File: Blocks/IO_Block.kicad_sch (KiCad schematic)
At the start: 0 parts

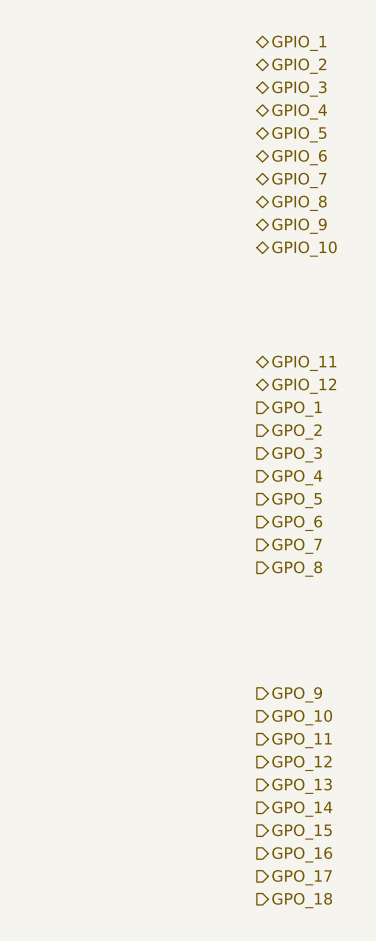
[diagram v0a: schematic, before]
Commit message: something
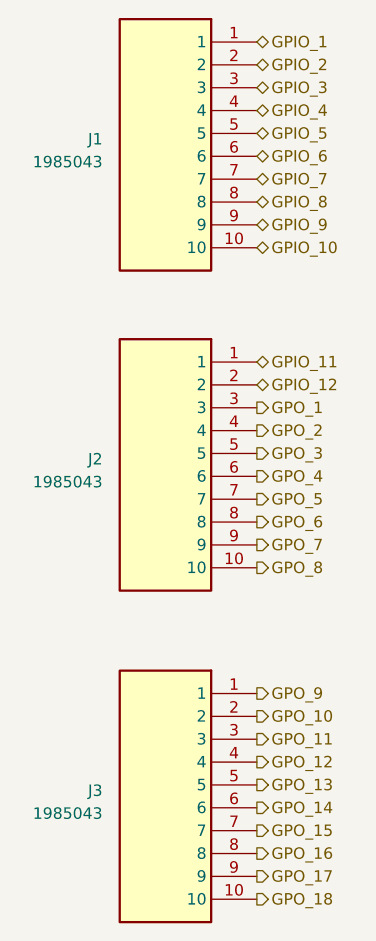
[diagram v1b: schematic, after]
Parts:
- added J1, J2, J3: 1985043, 1985043:1985043, symbol 1985043.kicad_sym:1985043
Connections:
- net GPIO_1: now also J1.1
- net GPIO_10: now also J1.10
- net GPIO_11: now also J2.1
- net GPIO_12: now also J2.2
- net GPIO_2: now also J1.2
- net GPIO_3: now also J1.3
- net GPIO_4: now also J1.4
- net GPIO_5: now also J1.5
- net GPIO_6: now also J1.6
- net GPIO_7: now also J1.7
- net GPIO_8: now also J1.8
- net GPIO_9: now also J1.9
- net GPO_1: now also J2.3
- net GPO_10: now also J3.2
- net GPO_11: now also J3.3
- net GPO_12: now also J3.4
- net GPO_13: now also J3.5
- net GPO_14: now also J3.6
- net GPO_15: now also J3.7
- net GPO_16: now also J3.8
- net GPO_17: now also J3.9
- net GPO_18: now also J3.10
- net GPO_2: now also J2.4
- net GPO_3: now also J2.5
- net GPO_4: now also J2.6
- net GPO_5: now also J2.7
- net GPO_6: now also J2.8
- net GPO_7: now also J2.9
- net GPO_8: now also J2.10
- net GPO_9: now also J3.1
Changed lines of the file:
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@@
     (effects (font (size 1.27 1.27)) (justify left))
   )
+  (symbol (lib_id "1985043.kicad_sym:1985043") (at 86.36 130.81 0) (mirror y) (unit 1)
+    (in_bom yes) (on_board yes) (dnp no)
+    (property "Reference" "J3" (at 69.215 141.605 0)
+      (effects (font (size 1.27 1.27)) (justify left))
+    )
+    (property "Value" "1985043" (at 69.215 144.145 0)
+      (effects (font (size 1.27 1.27)) (justify left))
+    )
+    (property "Footprint" "1985043:1985043" (at 69.85 225.73 0)
+      (effects (font (size 1.27 1.27)) (justify left top) hide)
+    )
+    (property "Datasheet" "https://www.phoenixcontact.com/online/portal/us/?uri=pxc-oc-itemdetail:pid=1985043&library=usen&pcck=P-11-01-05&tab=1&selectedCategory=ALL" (at 69.85 325.73 0)
+      (effects (font (size 1.27 1.27)) (justify left top) hide)
+    )
+    (property "Height" "13.1" (at 69.85 525.73 0)
+      (effects (font (size 1.27 1.27)) (justify left top) hide)
+    )
+    (property "Mouser Part Number" "651-1985043" (at 69.85 625.73 0)
+      (effects (font (size 1.27 1.27)) (justify left top) hide)
+    )
+    (property "Mouser Price/Stock" "https://www.mouser.co.uk/ProductDetail/Phoenix-Contact/1985043?qs=gjk32EaArKJe8oo3YkKpaw%3D%3D" (at 69.85 725.73 0)
+      (effects (font (size 1.27 1.27)) (justify left top) hide)
+    )
+    (property "Manufacturer_Name" "Phoenix Contact" (at 69.85 825.73 0)
+      (effects (font (size 1.27 1.27)) (justify left top) hide)
+    )
+    (property "Manufacturer_Part_Number" "1985043" (at 69.85 925.73 0)
+      (effects (font (size 1.27 1.27)) (justify left top) hide)
+    )
+    (pin "1")
+    (pin "10")
+    (pin "2")
+    (pin "3")
+    (pin "4")
+    (pin "5")
+    (pin "6")
+    (pin "7")
+    (pin "8")
+    (pin "9")
+    (instances
+      (project "PLC-CIM"
+        (path "/98f81d77-8880-491b-a7cf-4c27e2d73edf/ef38368d-af5e-44c5-8106-4a2f4dcc6c35"
+          (reference "J3") (unit 1)
+        )
+      )
+    )
+  )
+  (symbol (lib_id "1985043.kicad_sym:1985043") (at 86.36 58.42 0) (mirror y) (unit 1)
+    (in_bom yes) (on_board yes) (dnp no)
+    (property "Reference" "J1" (at 69.215 69.215 0)
+      (effects (font (size 1.27 1.27)) (justify left))
+    )
+    (property "Value" "1985043" (at 69.215 71.755 0)
+      (effects (font (size 1.27 1.27)) (justify left))
+    )
+    (property "Footprint" "1985043:1985043" (at 69.85 153.34 0)
+      (effects (font (size 1.27 1.27)) (justify left top) hide)
+    )
+    (property "Datasheet" "https://www.phoenixcontact.com/online/portal/us/?uri=pxc-oc-itemdetail:pid=1985043&library=usen&pcck=P-11-01-05&tab=1&selectedCategory=ALL" (at 69.85 253.34 0)
+      (effects (font (size 1.27 1.27)) (justify left top) hide)
+    )
+    (property "Height" "13.1" (at 69.85 453.34 0)
+      (effects (font (size 1.27 1.27)) (justify left top) hide)
+    )
+    (property "Mouser Part Number" "651-1985043" (at 69.85 553.34 0)
+      (effects (font (size 1.27 1.27)) (justify left top) hide)
+    )
+    (property "Mouser Price/Stock" "https://www.mouser.co.uk/ProductDetail/Phoenix-Contact/1985043?qs=gjk32EaArKJe8oo3YkKpaw%3D%3D" (at 69.85 653.34 0)
+      (effects (font (size 1.27 1.27)) (justify left top) hide)
+    )
+    (property "Manufacturer_Name" "Phoenix Contact" (at 69.85 753.34 0)
+      (effects (font (size 1.27 1.27)) (justify left top) hide)
+    )
+    (property "Manufacturer_Part_Number" "1985043" (at 69.85 853.34 0)
+      (effects (font (size 1.27 1.27)) (justify left top) hide)
+    )
+    (pin "1")
+    (pin "10")
+    (pin "2")
+    (pin "3")
+    (pin "4")
+    (pin "5")
+    (pin "6")
+    (pin "7")
+    (pin "8")
+    (pin "9")
+    (instances
+      (project "PLC-CIM"
+        (path "/98f81d77-8880-491b-a7cf-4c27e2d73edf/ef38368d-af5e-44c5-8106-4a2f4dcc6c35"
+          (reference "J1") (unit 1)
+        )
+      )
+    )
+  )
+  (symbol (lib_id "1985043.kicad_sym:1985043") (at 86.36 93.98 0) (mirror y) (unit 1)
+    (in_bom yes) (on_board yes) (dnp no)
+    (property "Reference" "J2" (at 69.215 104.775 0)
+      (effects (font (size 1.27 1.27)) (justify left))
+    )
+    (property "Value" "1985043" (at 69.215 107.315 0)
+      (effects (font (size 1.27 1.27)) (justify left))
+    )
+    (property "Footprint" "1985043:1985043" (at 69.85 188.9 0)
+      (effects (font (size 1.27 1.27)) (justify left top) hide)
+    )
+    (property "Datasheet" "https://www.phoenixcontact.com/online/portal/us/?uri=pxc-oc-itemdetail:pid=1985043&library=usen&pcck=P-11-01-05&tab=1&selectedCategory=ALL" (at 69.85 288.9 0)
+      (effects (font (size 1.27 1.27)) (justify left top) hide)
+    )
+    (property "Height" "13.1" (at 69.85 488.9 0)
+      (effects (font (size 1.27 1.27)) (justify left top) hide)
+    )
+    (property "Mouser Part Number" "651-1985043" (at 69.85 588.9 0)
+      (effects (font (size 1.27 1.27)) (justify left top) hide)
+    )
+    (property "Mouser Price/Stock" "https://www.mouser.co.uk/ProductDetail/Phoenix-Contact/1985043?qs=gjk32EaArKJe8oo3YkKpaw%3D%3D" (at 69.85 688.9 0)
+      (effects (font (size 1.27 1.27)) (justify left top) hide)
+    )
+    (property "Manufacturer_Name" "Phoenix Contact" (at 69.85 788.9 0)
+      (effects (font (size 1.27 1.27)) (justify left top) hide)
+    )
+    (property "Manufacturer_Part_Number" "1985043" (at 69.85 888.9 0)
+      (effects (font (size 1.27 1.27)) (justify left top) hide)
+    )
+    (pin "1")
+    (pin "10")
+    (pin "2")
+    (pin "3")
+    (pin "4")
+    (pin "5")
+    (pin "6")
+    (pin "7")
+    (pin "8")
+    (pin "9")
+    (instances
+      (project "PLC-CIM"
+        (path "/98f81d77-8880-491b-a7cf-4c27e2d73edf/ef38368d-af5e-44c5-8106-4a2f4dcc6c35"
+          (reference "J2") (unit 1)
+        )
+      )
+    )
+  )
 )
